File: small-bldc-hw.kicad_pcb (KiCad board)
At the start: 4 copper layers, 65 x 22.4 mm, 98 parts, among them J1 More IO, J2 TEMP, J3 CONN_01X01, J4 CONN_01X01, J5 CONN_01X01, J6 CAN, J7 I2C, J8 CONN_01X01, J9 CONN_01X01, P2 SWD, Q1 BUK7K13-60E, Q2 BUK7K13-60E, Q3 BUK7K13-60E, U1 STM32F042C6T6, U2 AZ1117C, U3 DRV8301, U4 MCP2562-E/SN, Y1 16MHz

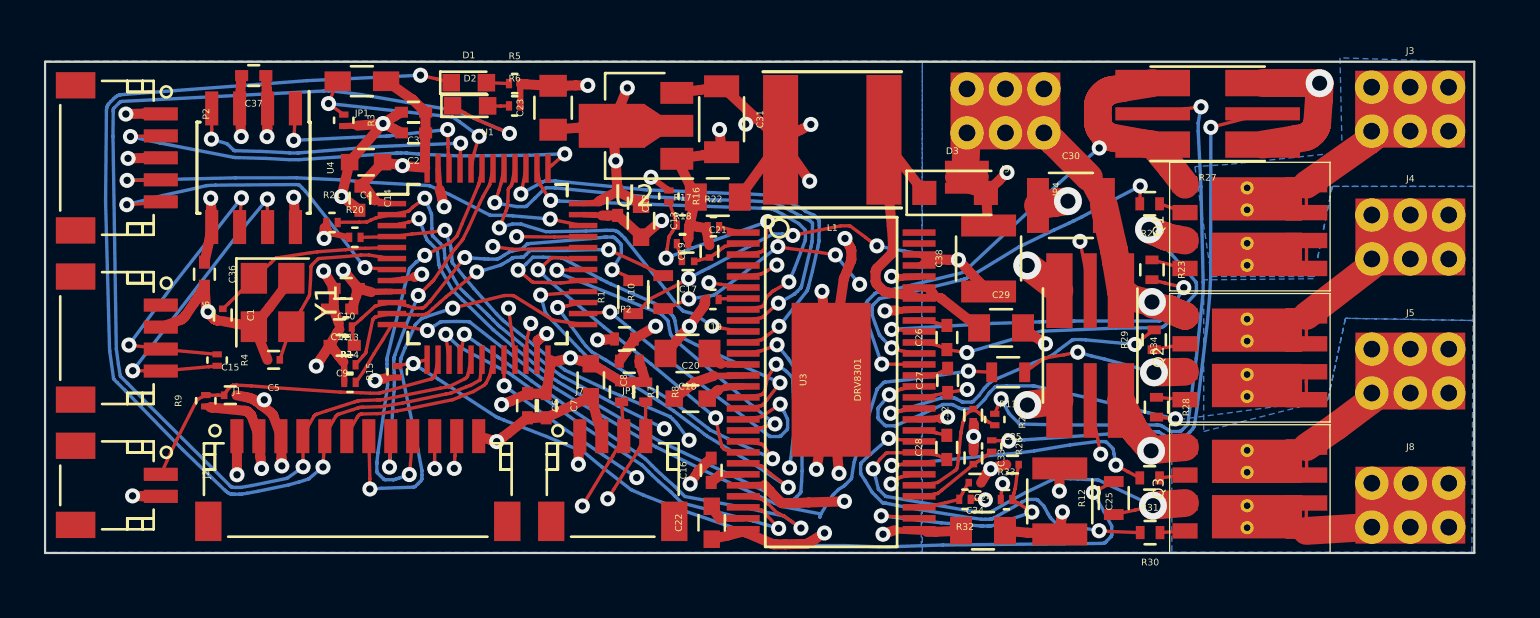
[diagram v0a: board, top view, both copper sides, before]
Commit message: all planes done
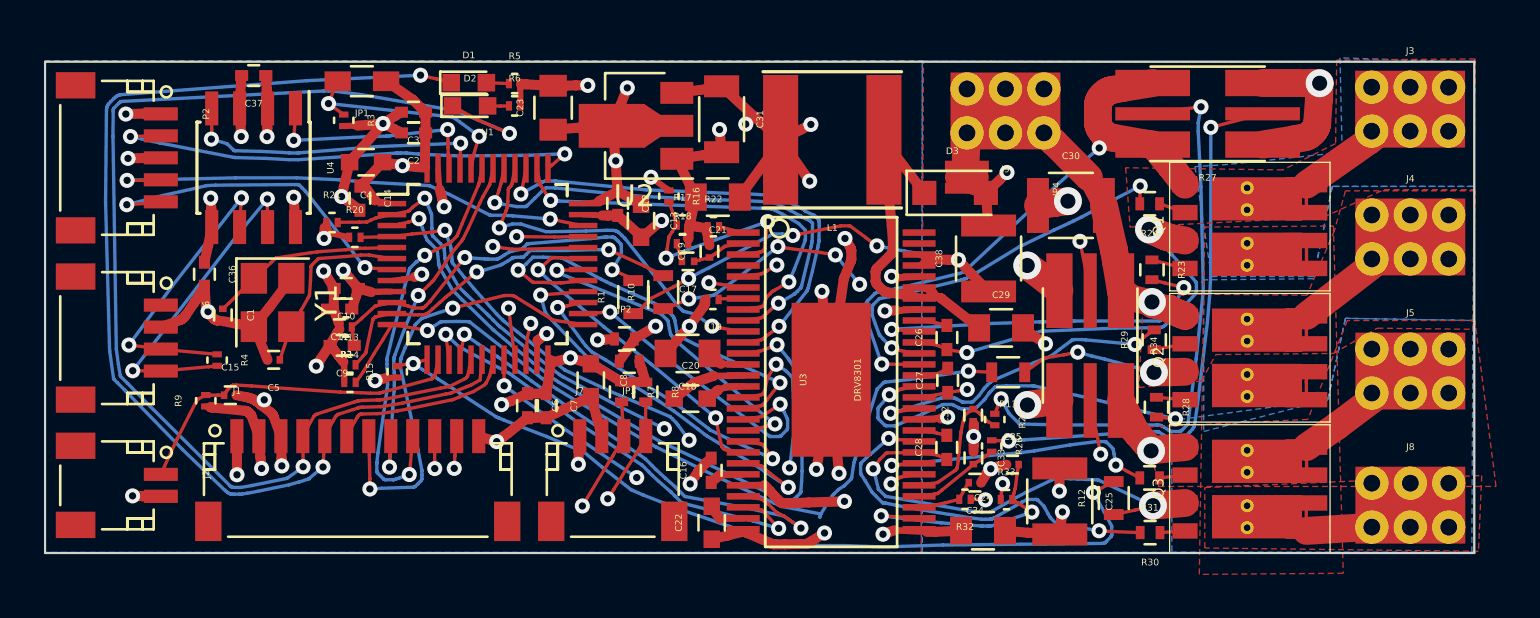
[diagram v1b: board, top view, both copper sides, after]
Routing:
- added copper zone on F.Cu, net /power/PHASE_A
- added copper zone on F.Cu, net /power/PHASE_B
- added copper zone on F.Cu, net /power/PHASE_C
- added copper zone on F.Cu, net DC_SUPPLY
- added copper zone on In2.Cu, net DC_SUPPLY
- added copper zone on F.Cu, net GND
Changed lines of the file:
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@@
   (layers
     (0 F.Cu signal)
-    (1 In1.Cu signal)
-    (2 In2.Cu signal)
-    (31 B.Cu signal)
+    (1 In1.Cu signal hide)
+    (2 In2.Cu signal hide)
+    (31 B.Cu signal hide)
     (35 F.Paste user)
     (36 B.SilkS user)
@@
       (pts
         (xy 178.6 89.7) (xy 178.6 94.3) (xy 169.9 94.3) (xy 169.9 100.2) (xy 172.8 100.2)
-        (xy 176.5 100.2) (xy 178.6 99.5) (xy 179.1 95.6) (xy 179.9 95.4) (xy 184.8 95.4)
+        (xy 176.1 99.15) (xy 177.4 97.55) (xy 179.1 95.6) (xy 179.9 95.4) (xy 184.8 95.4)
         (xy 184.8 89.8)
       )
@@
     (polygon
       (pts
-        (xy 184.9 95.6) (xy 179.2 95.6) (xy 178.4 100.2) (xy 171 100.3) (xy 170.9 102.6)
-        (xy 169.8 102.6) (xy 169.8 106.3) (xy 178.5 106.1) (xy 179 101.5) (xy 184.9 101.5)
+        (xy 184.9 95.6) (xy 179.2 95.6) (xy 176.65 98.05) (xy 171 100.3) (xy 170.9 102.6)
+        (xy 169.8 102.6) (xy 169.8 106.3) (xy 176.65 103.5) (xy 179 101.5) (xy 184.9 101.5)
         (xy 184.9 94.8)
       )
@@
     (polygon
       (pts
-        (xy 169.8 106.3) (xy 169.8 112) (xy 179 112) (xy 179 107.6) (xy 184.7 107.6)
-        (xy 184.9 101.5) (xy 179 101.5) (xy 178.4 106.3)
+        (xy 169.8 106.3) (xy 169.8 112) (xy 173 112) (xy 173.7 109) (xy 184.7 107.6)
+        (xy 184.9 101.5) (xy 179 101.5) (xy 177 103.7)
       )
     )
@@
       )
     )
+  )
+  (zone (net 2) (net_name GND) (layer F.Cu) (hatch edge 0.508)
+    (priority 1)
+    (connect_pads yes (clearance 0.508))
+    (min_thickness 0.254)
+    (fill yes (arc_segments 16) (thermal_gap 0.508) (thermal_bridge_width 0.508))
+    (polygon
+      (pts
+        (xy 159.85 89.7) (xy 119.9 89.7) (xy 119.9 112.1) (xy 159.75 112.1)
+      )
+    )
+  )
+  (zone (net 16) (net_name /power/PHASE_A) (layer F.Cu) (hatch edge 0.508)
+    (priority 5)
+    (connect_pads yes (clearance 0.508))
+    (min_thickness 0.254)
+    (fill yes (arc_segments 16) (thermal_gap 0.508) (thermal_bridge_width 0.508))
+    (polygon
+      (pts
+        (xy 184.95 89.6) (xy 178.65 89.65) (xy 178.6 93.45) (xy 176.2 94.65) (xy 169.05 94.55)
+        (xy 169.25 97.25) (xy 178.05 96.8) (xy 180.8 95.55) (xy 184.9 95.55)
+      )
+    )
+  )
+  (zone (net 18) (net_name /power/PHASE_B) (layer F.Cu) (hatch edge 0.508)
+    (priority 4)
+    (connect_pads yes (clearance 0.508))
+    (min_thickness 0.254)
+    (fill yes (arc_segments 16) (thermal_gap 0.508) (thermal_bridge_width 0.508))
+    (polygon
+      (pts
+        (xy 184.95 95.6) (xy 179.05 95.6) (xy 178.55 97.4) (xy 177.3 100.35) (xy 172.15 100.3)
+        (xy 169.85 100.5) (xy 169.65 104.55) (xy 172.5 104.25) (xy 173.15 103.05) (xy 178.5 103)
+        (xy 180.5 101.85) (xy 184.85 101.9)
+      )
+    )
+  )
+  (zone (net 15) (net_name DC_SUPPLY) (layer In2.Cu) (hatch edge 0.508)
+    (priority 1)
+    (connect_pads yes (clearance 0.508))
+    (min_thickness 0.254)
+    (fill yes (arc_segments 16) (thermal_gap 0.508) (thermal_bridge_width 0.508))
+    (polygon
+      (pts
+        (xy 185 107.9) (xy 173.1 109.05) (xy 173 112.05) (xy 184.9 112.05)
+      )
+    )
+  )
+  (zone (net 20) (net_name /power/PHASE_C) (layer F.Cu) (hatch edge 0.508)
+    (priority 6)
+    (connect_pads yes (clearance 0.508))
+    (min_thickness 0.254)
+    (fill yes (arc_segments 16) (thermal_gap 0.508) (thermal_bridge_width 0.508))
+    (polygon
+      (pts
+        (xy 184.934777 101.5) (xy 179.134777 101.5) (xy 177.334777 106) (xy 169.984777 106.35) (xy 170.55 109.05)
+        (xy 185.9 109.05)
+      )
+    )
+  )
+  (zone (net 15) (net_name DC_SUPPLY) (layer F.Cu) (hatch edge 0.508)
+    (priority 5)
+    (connect_pads yes (clearance 0.508))
+    (min_thickness 0.254)
+    (fill yes (arc_segments 16) (thermal_gap 0.508) (thermal_bridge_width 0.508))
+    (polygon
+      (pts
+        (xy 185.1 112) (xy 172.65 111.85) (xy 172.65 109.1) (xy 185.25 108.55)
+      )
+    )
+  )
+  (zone (net 15) (net_name DC_SUPPLY) (layer F.Cu) (hatch edge 0.508)
+    (priority 1)
+    (connect_pads yes (clearance 0.508))
+    (min_thickness 0.254)
+    (fill yes (arc_segments 16) (thermal_gap 0.508) (thermal_bridge_width 0.508))
+    (polygon
+      (pts
+        (xy 172.65 97.25) (xy 178.5 97.2) (xy 178.95 113) (xy 172.4 113.05)
+      )
+    )
